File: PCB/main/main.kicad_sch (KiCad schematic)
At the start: 4 parts, among them J1 Conn_01x33_Female, J2 Conn_01x33_Female, J3 Conn_01x33_Female, J4 Conn_01x33_Female

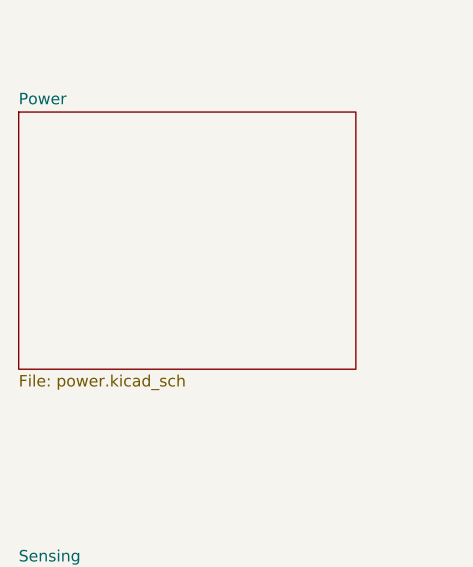
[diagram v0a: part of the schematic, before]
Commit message: Power Module v0.02
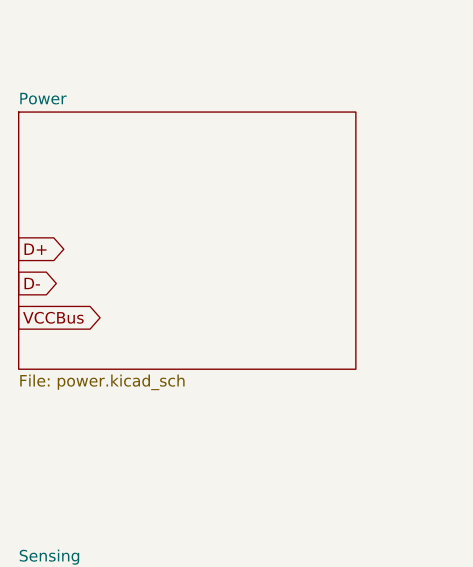
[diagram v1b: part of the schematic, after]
